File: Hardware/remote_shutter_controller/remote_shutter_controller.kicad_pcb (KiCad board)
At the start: 2 copper layers, 71 parts, among them J1 USB_C_Receptacle_USB2.0, J2 Switch, Q1 BC847BDW1, Q2 FDN335N, Q3 FDN338P, SW1 RotaryEncoder_Switch, U1 ESP32-PICO-MINI-02, U2 AZ1117-3.3, U3 L78L09_SOT89, U4 TP4056, U5 CP2102N-Axx-xQFN24, U6 X077-6428TSWCG01-H13, Y1 NX3215SA-32.768K-STD-MUA-14

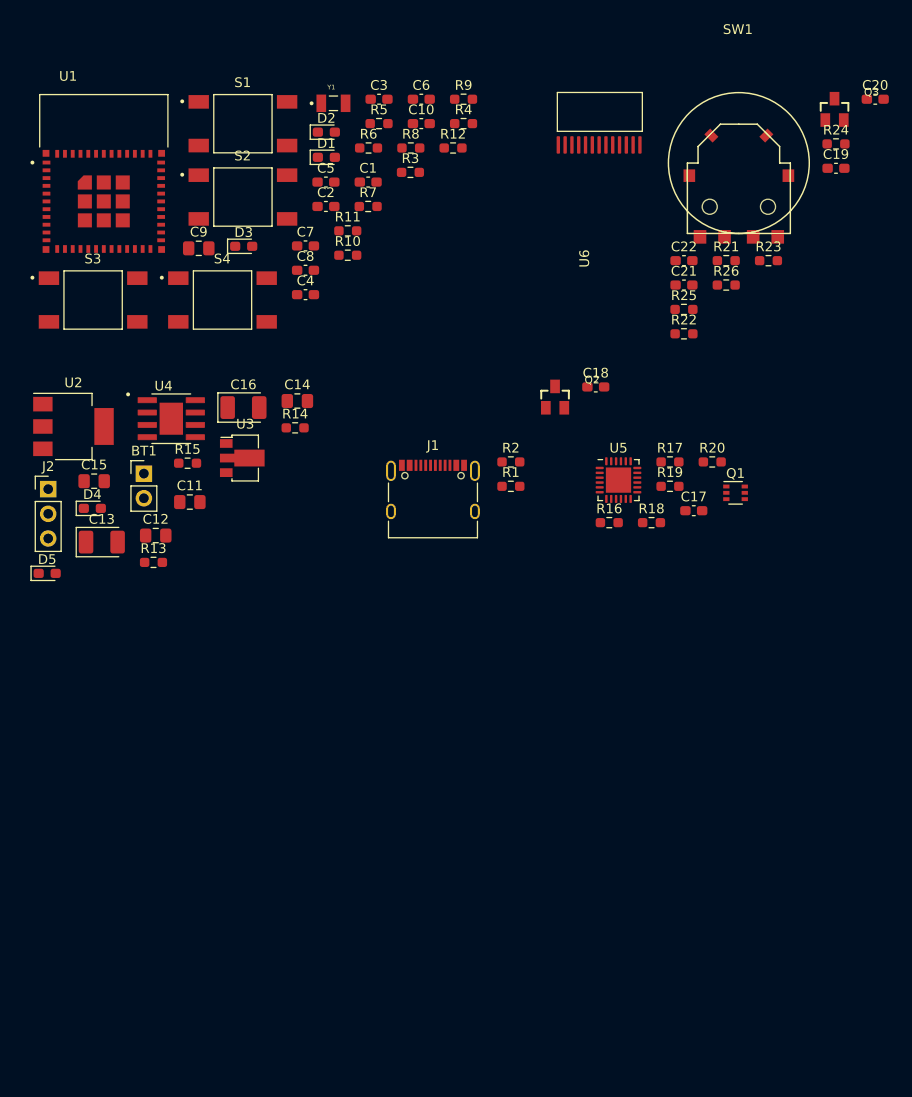
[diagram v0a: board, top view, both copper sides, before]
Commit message: Further layout work
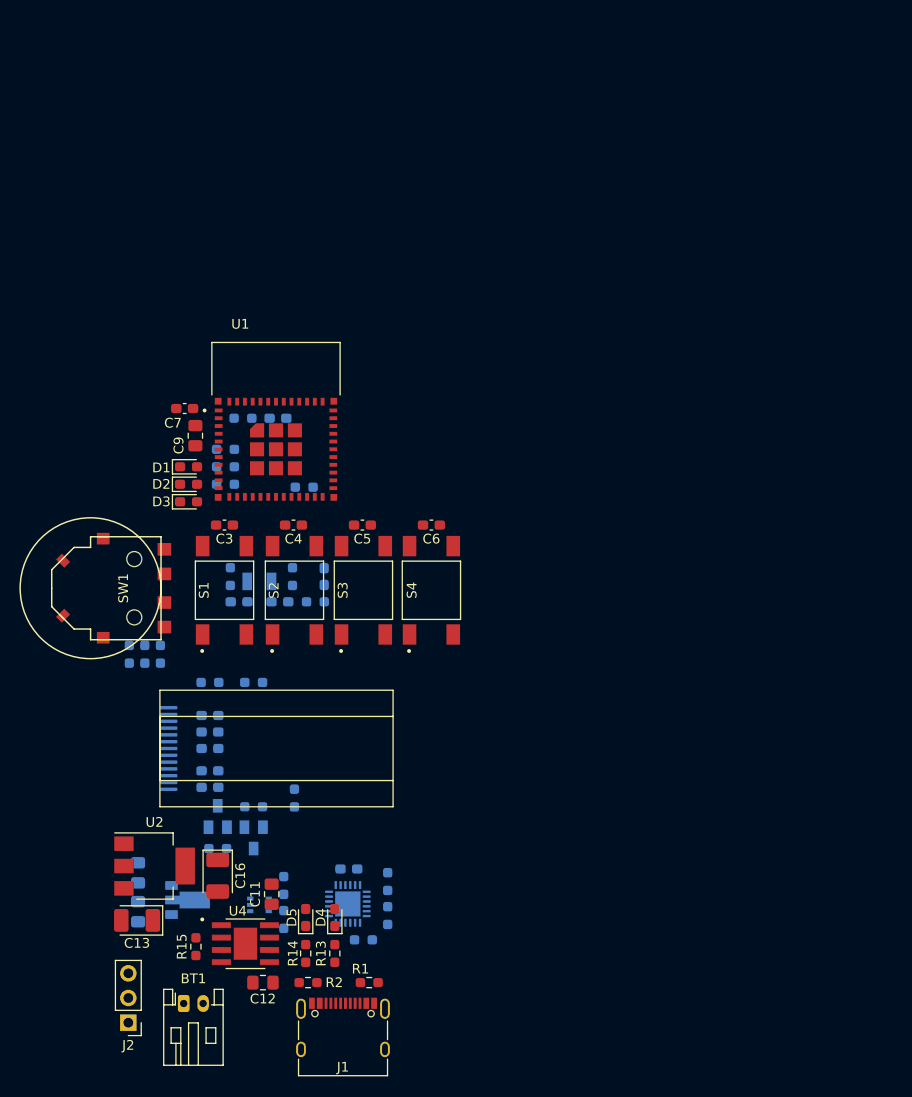
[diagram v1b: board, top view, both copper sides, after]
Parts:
- BT1: footprint Connector_PinHeader_2.54mm:PinHeader_1x02_P2.54mm_Vertical -> Connector_JST:JST_PH_S2B-PH-K_1x02_P2.00mm_Horizontal
- C1, C10, C14, C15, C17, C18, C19, C2, C20, C21, C22, C8, Q1, Q2, Q3, R10, R11, R12, R16, R17, R18, R19, R20, R21, R22, R23, R24, R25, R26, R3, R4, R5, R6, R7, R8, R9, U3, U5, U6, Y1: moved to B.Cu
- moved Q3 96.6 mm to (125.2, 133.2), turned to 180 degrees
- moved C20 95.7 mm to (124.4, 126.2)
- moved C19 90.6 mm to (124.4, 130.2), turned to 180 degrees
- moved R24 88.4 mm to (117.7, 116.5), turned to -90 degrees
- moved SW1 78.1 mm to (113.4, 109.7), turned to 90 degrees
- moved U6 77.6 mm to (119.2, 126.2), turned to -90 degrees
- moved R23 74.6 mm to (119.3, 116.5), turned to 90 degrees
- moved R21 74.3 mm to (128.9, 132.2)
- moved R22 71.5 mm to (125.2, 136.5)
- moved R26 69.0 mm to (133.1, 131.3), turned to -90 degrees
- moved C22 68.8 mm to (124.4, 124.5)
- moved R25 67.2 mm to (116.1, 116.5), turned to 90 degrees
- moved C21 65.9 mm to (124.4, 122.8)
- moved Q1 64.8 mm to (129.5, 142.3)
- moved R20 64.5 mm to (132.0, 143.8), turned to 90 degrees
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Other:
- copper layers 2 -> 4

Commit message: Layout pre-routing
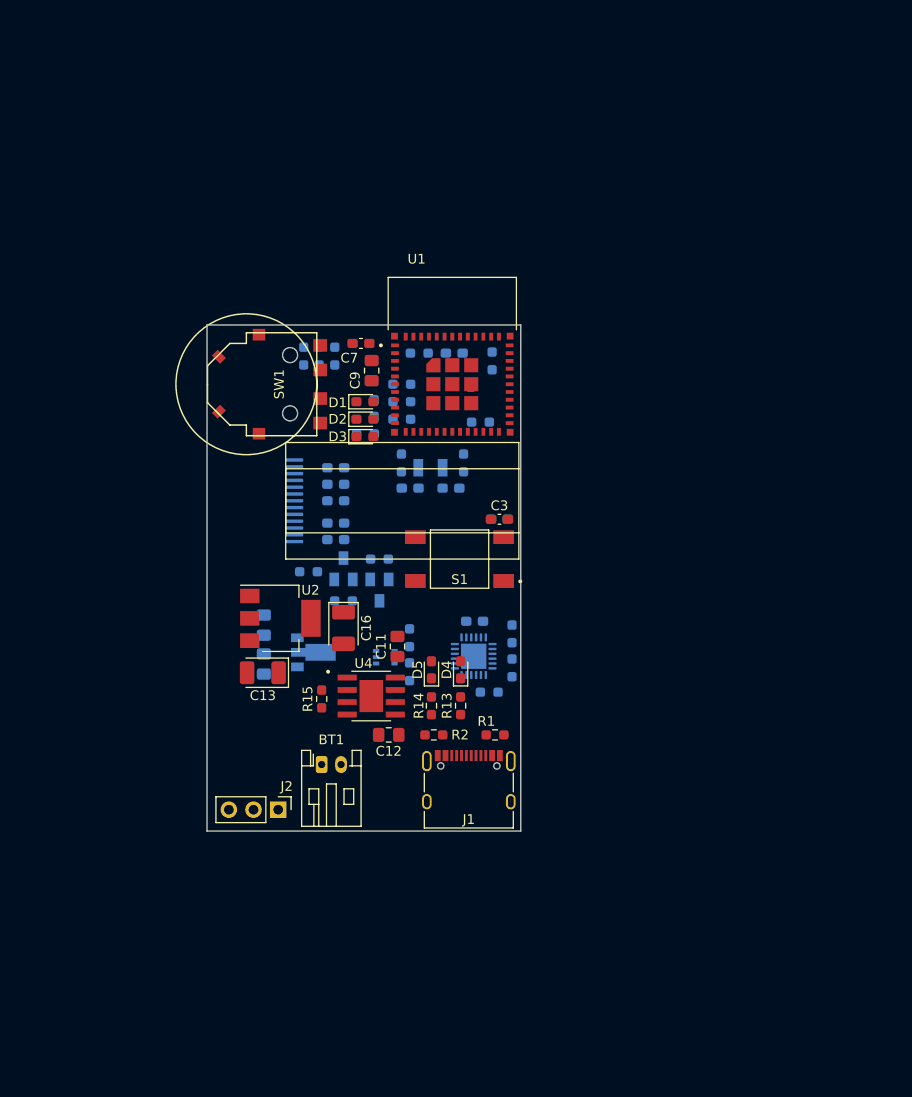
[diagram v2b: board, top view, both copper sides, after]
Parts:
- removed C5, C6: 0u1, Capacitor_SMD:C_0603_1608Metric_Pad1.08x0.95mm_HandSolder
- removed S3, S4: 4-1437565-2, footprint:SW_4-1437565-2
- C4, S2: moved to B.Cu
- moved R11 44.0 mm to (153.4, 86.3), turned to -90 degrees
- moved R12 37.0 mm to (151.2, 89.9), turned to -90 degrees
- moved R25 35.6 mm to (134.1, 85.8)
- moved R23 35.6 mm to (137.2, 85.8)
- moved R24 35.6 mm to (135.7, 85.8)
- moved C12 28.6 mm to (142.8, 124.8)
- moved R13 28.6 mm to (150.2, 121.8)
- moved R14 28.6 mm to (147.2, 121.8)
- moved U3 28.6 mm to (135.1, 116.3)
- moved C16 28.6 mm to (138.2, 113.8)
- moved U2 28.6 mm to (131.7, 112.8)
- moved Q1 28.6 mm to (142.4, 116.8)
- moved R1 28.6 mm to (153.8, 124.8)
- moved R19 28.6 mm to (144.9, 114.8)
- moved R2 28.6 mm to (147.4, 124.8)
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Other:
- board outline added: 32.3 x 52.1 mm

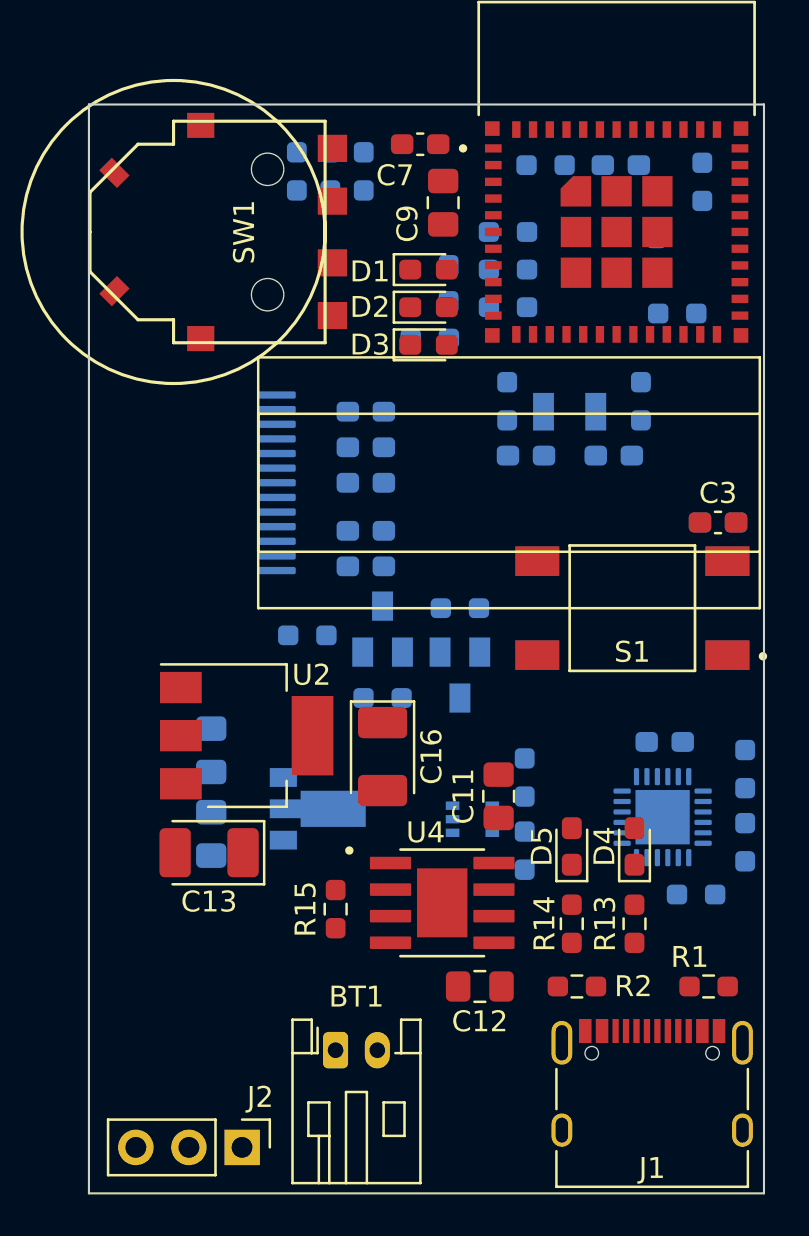
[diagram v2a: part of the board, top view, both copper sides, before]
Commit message: Initial routing.
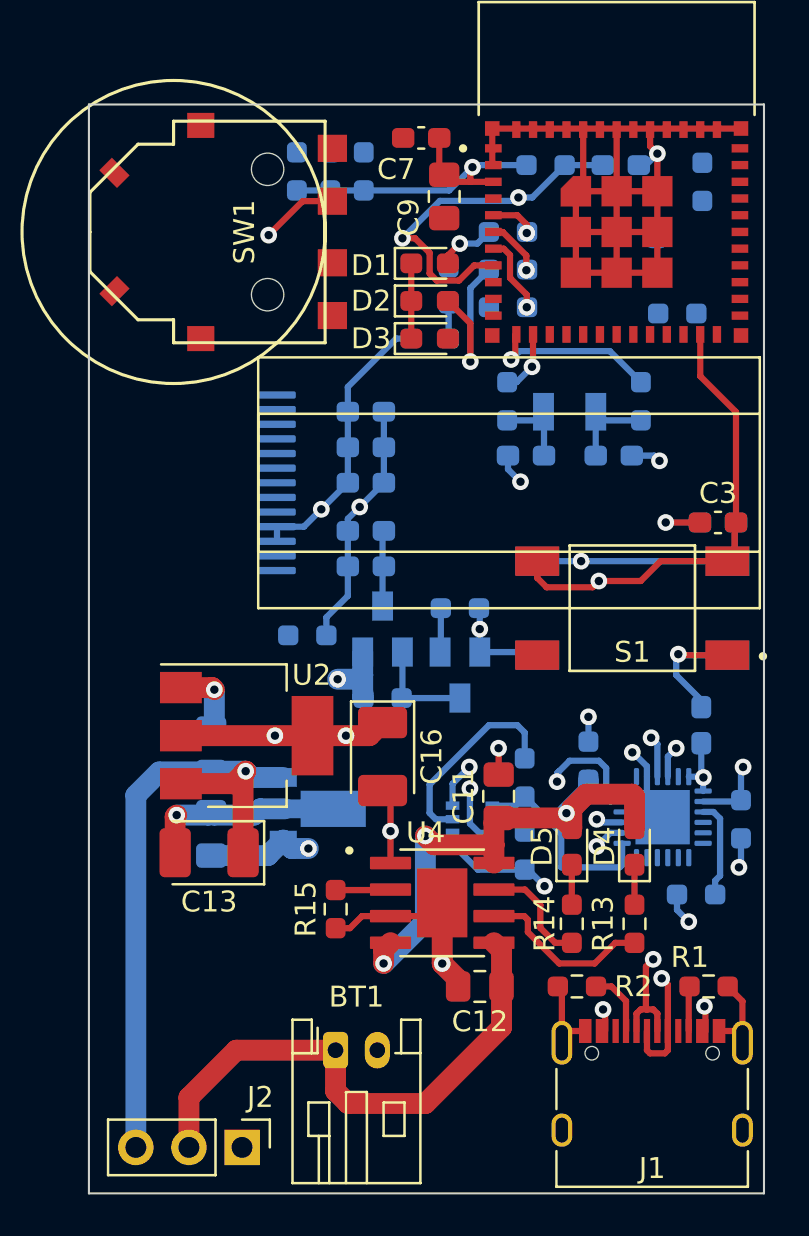
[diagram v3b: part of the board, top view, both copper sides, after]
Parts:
- moved R16 8.45 mm to (148.0, 114.0)
- moved R17 2.41 mm to (155.3, 116.8), turned to -90 degrees
- moved C17 1.92 mm to (153.4, 112.3), turned to 90 degrees
- moved C7 0.30 mm to (140.0, 84.2)
- moved D1 0.30 mm to (140.4, 90.2)
- moved D2 0.30 mm to (140.4, 92.0)
- moved D3 0.30 mm to (140.4, 93.8)
- moved C9 0.30 mm to (141.1, 87.0)
- turned R13 to -90 degrees
- turned R9 to -90 degrees
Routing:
- net GND: track 0.00 -> 125.0 mm, vias 0 -> 15
- net /MCU/EN: track 0.00 -> 61.1 mm, vias 0 -> 4
- net +3V3: track 0.00 -> 44.7 mm, vias 0 -> 6
- net /VBUS: track 0.00 -> 43.9 mm, vias 0 -> 5
- net /MCU/IO0: track 0.00 -> 39.9 mm, vias 0 -> 2
- net Net-(C13-Pad1): track 0.00 -> 31.8 mm, vias 0 -> 1
- net /Power/VBAT: track 0.00 -> 26.2 mm
- net /DP: track 0.00 -> 19.7 mm, vias 0 -> 2
- net /DN: track 0.00 -> 17.5 mm, vias 0 -> 2
- net /MCU/9V: track 0.00 -> 17.3 mm, vias 0 -> 2
- net /Comms/DTR: track 0.00 -> 16.4 mm, vias 0 -> 2
- net Net-(R16-Pad2): track 0.00 -> 13.2 mm, vias 0 -> 2
- net /Comms/RTS: track 0.00 -> 9.84 mm
- net Net-(Q1-Pad2): track 0.00 -> 9.69 mm
- net Net-(R13-Pad2): track 0.00 -> 8.42 mm
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- added copper zone on In2.Cu, net +3V3
- added copper zone on In1.Cu, net GND
